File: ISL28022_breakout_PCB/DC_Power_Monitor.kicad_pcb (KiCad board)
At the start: 2 copper layers, 59.9 x 54.9 mm, 21 parts, among them J1 DATA, J2 DATA, J3 ID_A0, J4 ID_A1, J5 PCB, J6 LOGO1, J7 LOGO2, J8 INPUT, J9 OUTPUT, U1 ISL28022

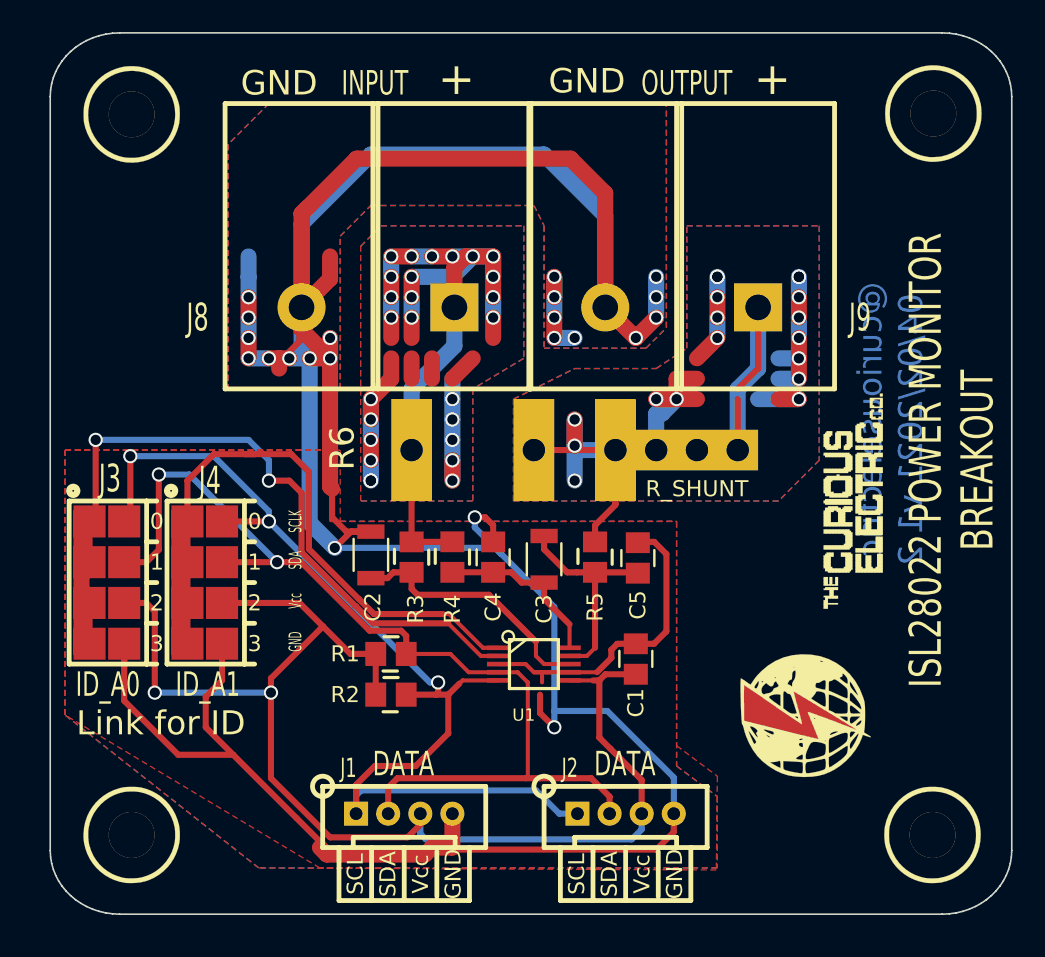
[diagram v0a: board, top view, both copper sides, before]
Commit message: updated instructions
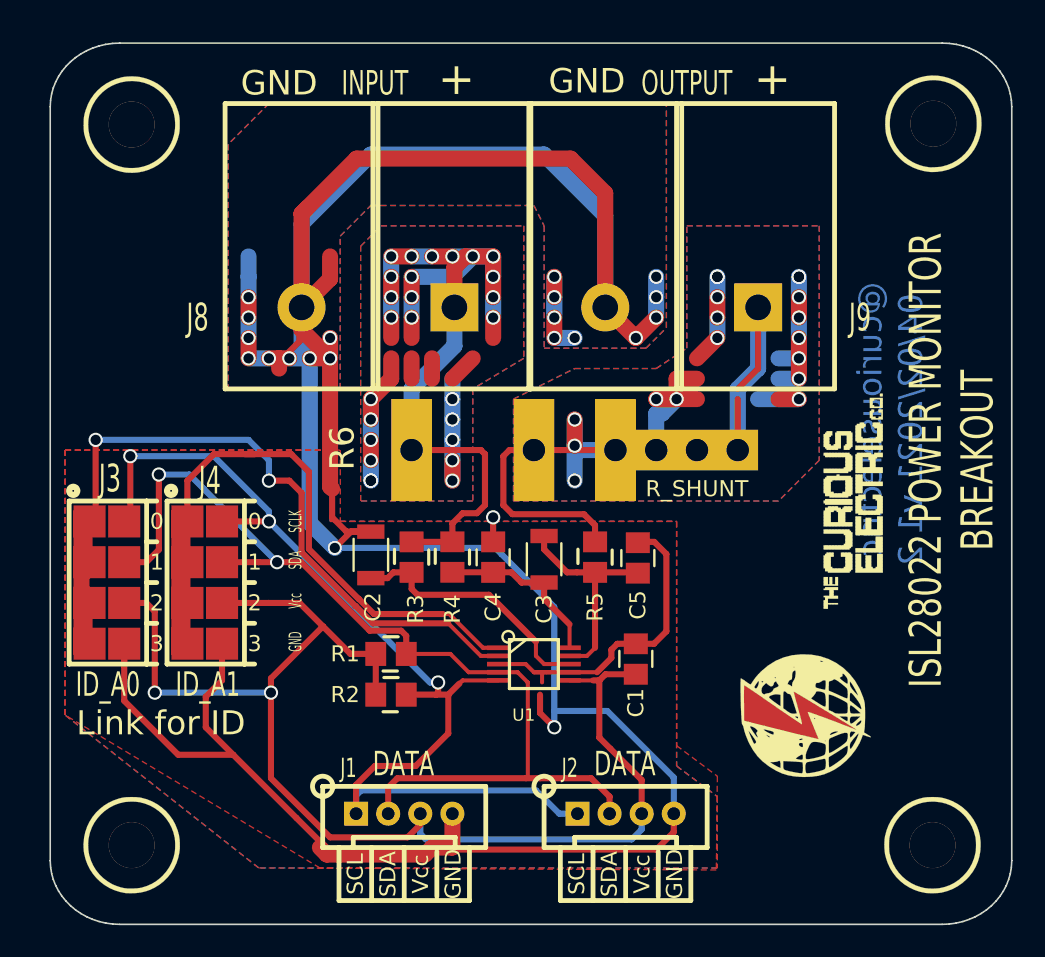
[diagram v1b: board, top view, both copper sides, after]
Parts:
- moved J5 0.64 mm to (83.7, 127.2)
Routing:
- net /Ishn: track 74.7 -> 80.8 mm
- net /Ishp: track 76.9 -> 82.7 mm
- net GND: track 281.2 -> 277.4 mm

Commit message: updated
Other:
- net class Default removed
